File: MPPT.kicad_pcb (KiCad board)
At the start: 2 copper layers, 125 x 150 mm, 133 parts, among them J1 Car Power, J2 Solar Array, J3 Battery, J4 CAN_In, J5 CAN_Out, Q1 NMOS, Q2 NMOS, SW1 RESET, SW2 SW_DIP_x02, U1 Nucleo_L432KC, U2 UCC37321, U3 PQMC3-D12-S9-S, U4 INA210, U5 INA210, U6 MAX40075AUT+, U7 MAX40075AUT+, U8 ADM3055E, U9 CDSOT23-T24CAN

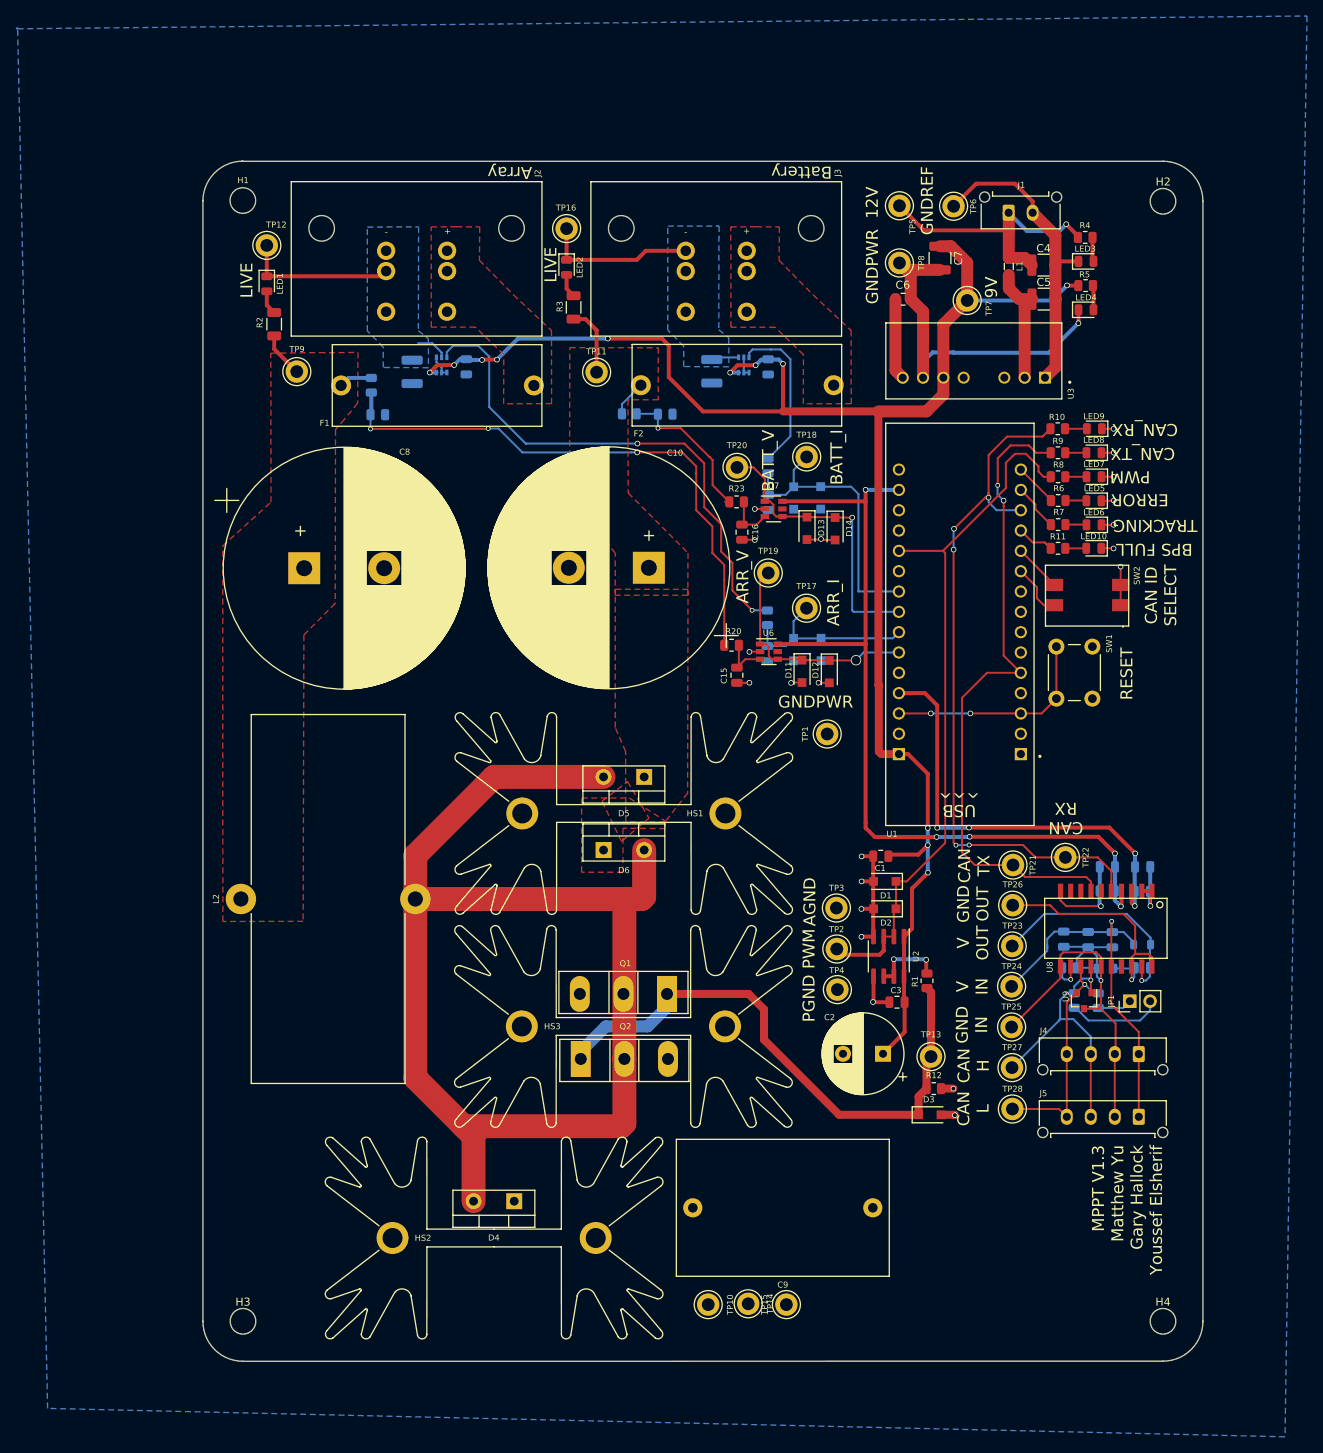
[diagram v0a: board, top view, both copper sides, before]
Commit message: Finalized board layout.
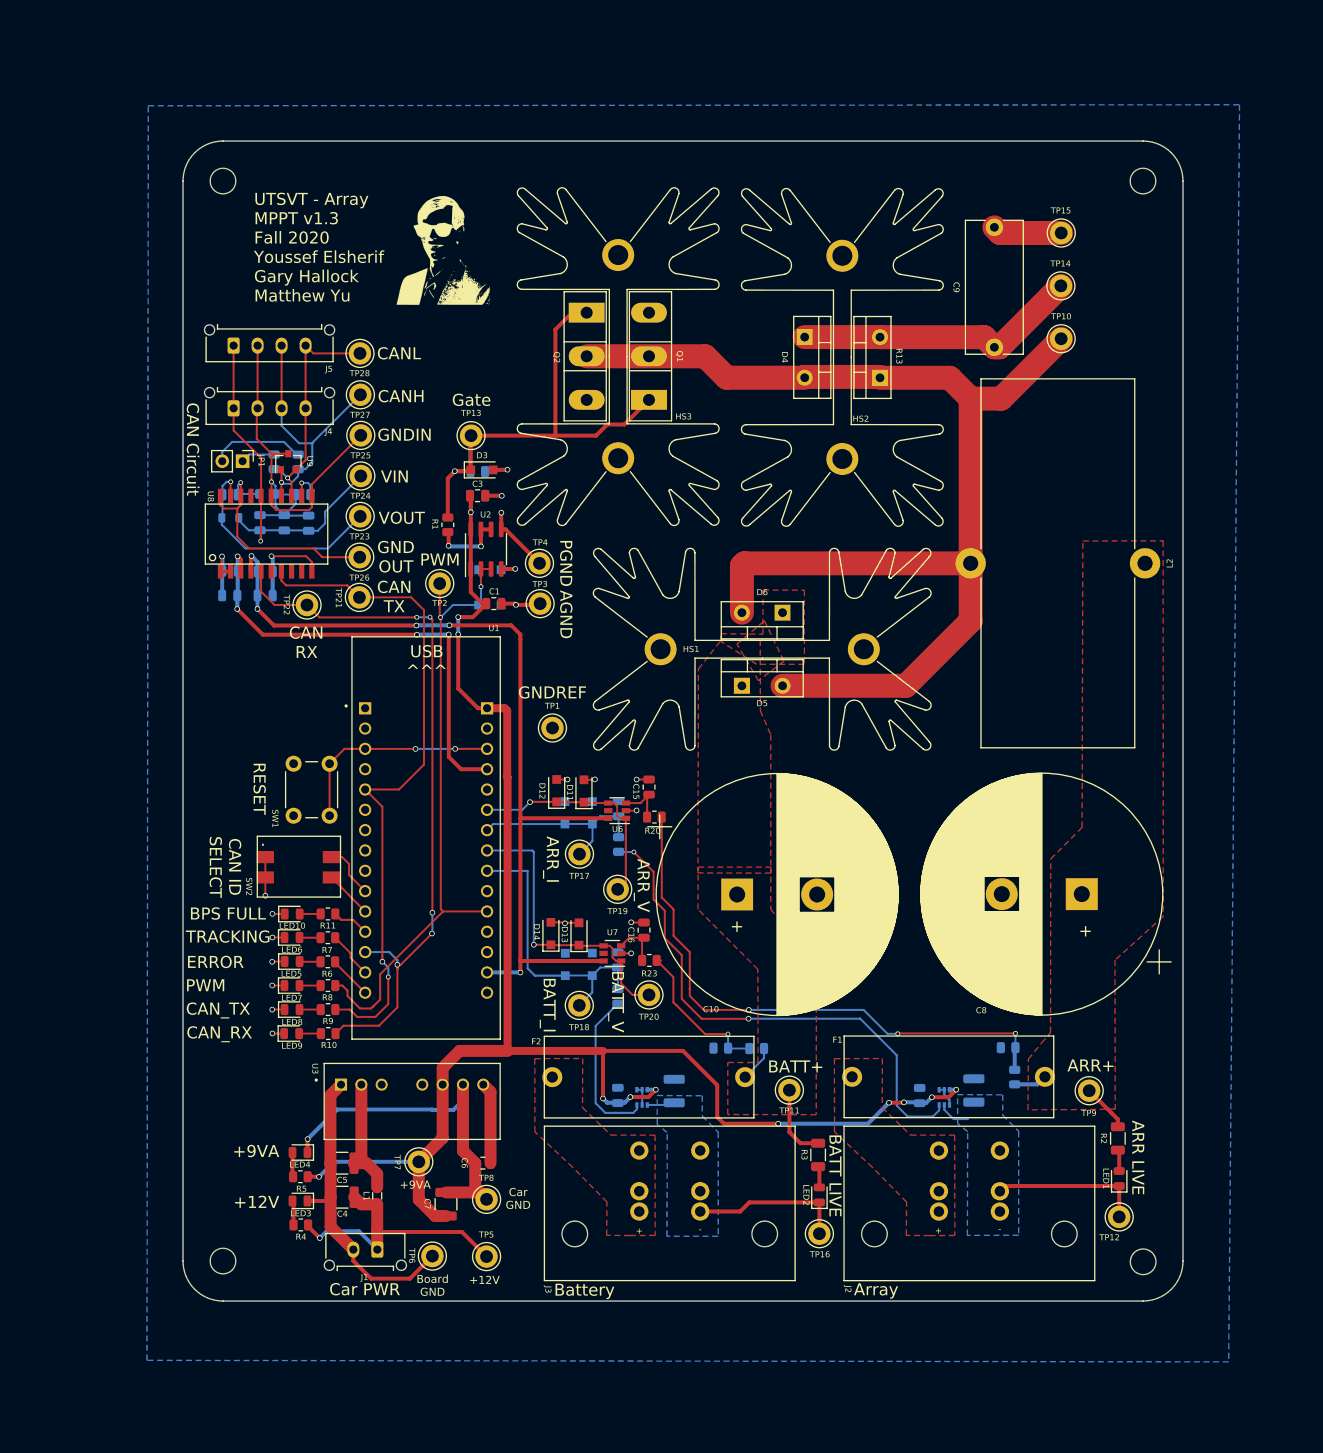
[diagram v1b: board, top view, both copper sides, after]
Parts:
- added G***: LOGO, UTSVT_Special:UTSVT_Logo_Symbol, B.Cu at (35.8, 27.7)
- added G***: LOGO, UTSVT_Special:Hallock_Image_Tiny, F.Cu at (49.5, 31.0)
- added R13: R, Package_TO_SOT_THT:TO-220-2_Vertical, F.Cu at (104.6, 47.1)
- C2: footprint Capacitor_THT:CP_Radial_D10.0mm_P5.00mm -> Capacitor_SMD:C_0805_2012Metric; moved to B.Cu
- C9: footprint MPPT_Custom:C_Rect_L26.5mm_W17.0mm_P22.50mm_MKS4 -> Capacitor_THT:C_Rect_L16.5mm_W7.0mm_P15.00mm_MKT
- D1, D2, R12: moved to B.Cu
- TP8: value GNDP -> Device GND
- moved H4 184.7 mm to (22.5, 22.5), turned to 180 degrees
- moved H3 181.6 mm to (137.5, 22.5), turned to 180 degrees
- moved H2 177.1 mm to (22.5, 157.5), turned to 180 degrees
- moved H1 173.8 mm to (137.5, 157.5), turned to 180 degrees
- moved TP12 161.6 mm to (134.5, 152.0), turned to 0 degrees
- moved R4 157.6 mm to (32.2, 153.0), turned to 0 degrees
- moved LED1 154.5 mm to (134.5, 147.2), turned to 90 degrees
- moved LED3 153.1 mm to (32.1, 150.0), turned to 180 degrees
- moved J1 151.7 mm to (41.8, 156.0), turned to 180 degrees
- moved J5 148.6 mm to (23.8, 43.0), turned to 0 degrees
- moved R5 148.5 mm to (32.2, 146.9), turned to 0 degrees
- moved R2 146.6 mm to (134.4, 142.1), turned to 90 degrees
- moved TP6 146.5 mm to (48.7, 156.8), turned to 90 degrees
- moved C4 145.8 mm to (37.4, 149.5), turned to 180 degrees
- moved LED4 144.0 mm to (32.1, 143.9), turned to 180 degrees
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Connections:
- C1 pad 1: GNDPWR -> GNDREF
- C10 pad 2: GNDPWR -> GNDREF
- C11 pad 2: GNDPWR -> GNDREF
- C12 pad 2: GNDPWR -> GNDREF
- C13 pad 2: GNDPWR -> GNDREF
- C14 pad 2: GNDPWR -> GNDREF
- C15 pad 2: GNDPWR -> GNDREF
- C16 pad 2: GNDPWR -> GNDREF
- C17 pad 2: GNDPWR -> GNDREF
- C18 pad 2: GNDPWR -> GNDREF
- C19 pad 2: GNDPWR -> GNDREF
- C2 pad 2: GNDPWR -> GNDREF
- C20 pad 2: GNDPWR -> GNDREF
- C3 pad 2: GNDPWR -> GNDREF
- C4 pad 2: GNDREF -> GNDPWR
- C5 pad 2: GNDREF -> GNDPWR
- C6 pad 1: GNDPWR -> GNDREF
- C7 pad 2: GNDPWR -> GNDREF
- C8 pad 2: GNDPWR -> GNDREF
- C9 pad 2: GNDPWR -> GNDREF
- D1 pad 2: GNDPWR -> GNDREF
- D10 pad 2: GNDPWR -> GNDREF
- D11 pad 2: GNDPWR -> GNDREF
- D12 pad 2: GNDPWR -> GNDREF
- D13 pad 2: GNDPWR -> GNDREF
- D14 pad 2: GNDPWR -> GNDREF
- D2 pad 2: GNDPWR -> GNDREF
- D3 pad 2: GNDPWR -> GNDREF
- D7 pad 2: GNDPWR -> GNDREF
- D8 pad 2: GNDPWR -> GNDREF
- D9 pad 2: GNDPWR -> GNDREF
- J1 pad 2: GNDREF -> GNDPWR
- LED10 pad 1: GNDPWR -> GNDREF
- LED3 pad 1: GNDREF -> GNDPWR
- LED4 pad 1: GNDPWR -> GNDREF
- LED5 pad 1: GNDPWR -> GNDREF
- LED6 pad 1: GNDPWR -> GNDREF
- LED7 pad 1: GNDPWR -> GNDREF
- LED8 pad 1: GNDPWR -> GNDREF
- LED9 pad 1: GNDPWR -> GNDREF
- Q1 pad 3: GNDPWR -> GNDREF
- Q2 pad 3: GNDPWR -> GNDREF
- R12 pad 2: GNDPWR -> GNDREF
- R14 pad 1: GNDPWR -> GNDREF
- R16 pad 2: GNDPWR -> GNDREF
- R19 pad 2: GNDPWR -> GNDREF
- R22 pad 2: GNDPWR -> GNDREF
- SW1 pad 2: GNDPWR -> GNDREF
- SW2 pad 1: GNDPWR -> GNDREF
- SW2 pad 2: GNDPWR -> GNDREF
- TP1 pad 1: GNDPWR -> GNDREF
- TP15 pad 1: GNDPWR -> GNDREF
- TP3 pad 1: GNDPWR -> GNDREF
- TP4 pad 1: GNDPWR -> GNDREF
- TP6 pad 1: GNDREF -> GNDPWR
- TP8 pad 1: GNDPWR -> GNDREF
- U1 pad 29: GNDPWR -> GNDREF
- U1 pad 4: GNDPWR -> GNDREF
- U2 pad 4: GNDPWR -> GNDREF
- U2 pad 5: GNDPWR -> GNDREF
- U3 pad 1: GNDREF -> GNDPWR
- U3 pad 7: GNDPWR -> GNDREF
- U4 pad 1: GNDPWR -> GNDREF
- U4 pad 2: GNDPWR -> GNDREF
- U4 pad 4: GNDPWR -> GNDREF
- U5 pad 1: GNDPWR -> GNDREF
- U5 pad 2: GNDPWR -> GNDREF
- U5 pad 5: GNDPWR -> GNDREF
- U6 pad 2: GNDPWR -> GNDREF
- U7 pad 2: GNDPWR -> GNDREF
- U8 pad 1: GNDPWR -> GNDREF
- U8 pad 10: GNDPWR -> GNDREF
- U8 pad 2: GNDPWR -> GNDREF
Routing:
- net GNDREF: track 38.8 -> 126.5 mm, vias 0 -> 22
- net GNDPWR: track 122.3 -> 38.8 mm, vias 24 -> 0
- net Net-(C9-Pad1): track 0.00 -> 35.7 mm
- net +9VA: track 218.0 -> 204.9 mm
- net /Drive_PWM: track 73.0 -> 61.2 mm, vias 0 -> 1
- net /PWM: track 88.6 -> 82.1 mm, vias 0 -> 2
- net Net-(D4-Pad2): track 156.7 -> 153.9 mm
- net /CAN_Tx: track 82.5 -> 84.2 mm
- net /CAN_Rx: track 88.6 -> 90.3 mm
- net +5V: track 55.5 -> 57.2 mm
- net +3V3: track 109.4 -> 111.1 mm
- net /+Batt: track 13.3 -> 14.0 mm
- added copper zone on B.Cu, net GNDREF
- removed copper zone on B.Cu, net GNDPWR
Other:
- board size 125 x 150 mm -> 125 x 145 mm
- board text added: "+12V"
- board text added: "+9VA"
- board text added: "ARR LIVE"
- board text added: "ARR+"
- board text added: "BATT LIVE"
- board text added: "BATT+"
- board text added: "Board GND"
- board text added: "CAN Circuit"
- board text added: "CANH"
- board text added: "CANL"
- board text added: "Car GND"
- board text added: "Car PWR"
- board text added: "GNDIN"
- board text added: "Gate"
- board text added: "In principle, I am concerned about routing thin analog signals across two power planes for high power systems. Especially in the case where the system is attempting to rapidly shift the voltage to maximize the current, sometimes in large steps, which may cause outsized current fluctuations and electromagnetic interference."
- board text added: "UTSVT - Array MPPT v1.3 Fall 2020 Youssef Elsherif Gary Hallock Matthew Yu"
- board text added: "VIN"
- board text added: "VOUT"
- board text removed: "12V"
- board text removed: "9V"
- board text removed: "CAN H"
- board text removed: "CAN L"
- board text removed: "GND IN"
- board text removed: "GNDPWR"
- board text removed: "I am concerned about routing thin analog signals across two power planes for high power systems. Especially where the MPPT is attempting to shift the voltage to maximize the current, sometimes in large steps."
- board text removed: "I don't like how this 9V line runs across multiple high power planes. Route from top?"
- board text removed: "I have concern about overlapping these sensor circuits.."
- board text removed: "I wonder if this voltage out of the divider is too close.."
- board text removed: "LIVE"
- board text removed: "Leave some space for metadata. Component sections should also have identifying labels. All chips or polarized components should be marked for positive/pin1."
- board text removed: "MPPT V1.3 Matthew Yu Gary Hallock Youssef Elsherif"
- board text removed: "Need to figure out what the possible snubber values could be and select a generic footprint to fit them."
- board text removed: "Should check again what the tolerances and padding should be around these components in the heatsink."
- board text removed: "V IN"
- board text removed: "V OUT"
- board text removed: "We can probably cut the layout down another 3-5% if we use smaller, more efficient heat sinks."
- board text removed: "uC might want to be moved over a little bit more and the 9V line expanded to 2mm and 1mm lines to CAN and Drive PWM."
